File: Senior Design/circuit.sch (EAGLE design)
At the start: 24 parts, among them IC1 74HC164N, IC2 ATMEGA328P, IC3 ATTINY24A, Q1 16 MHz

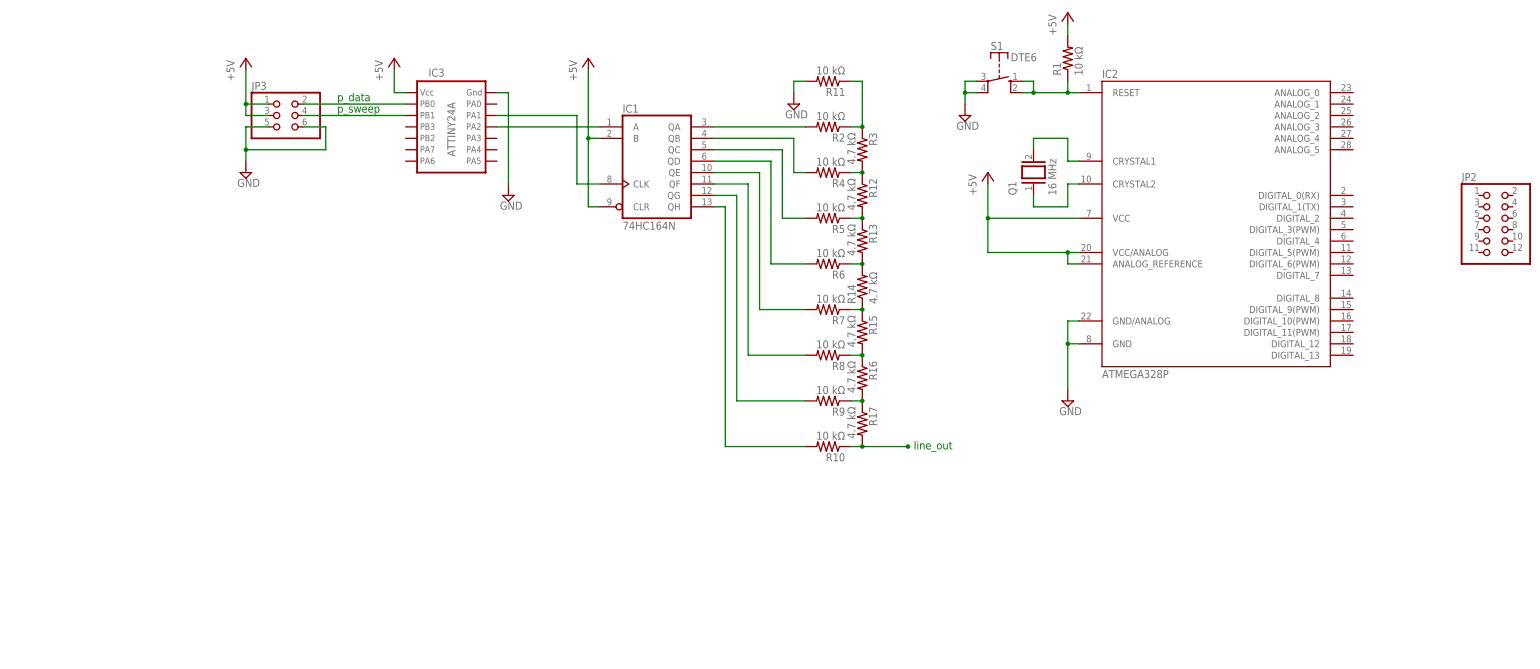
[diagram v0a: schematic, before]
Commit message: working on senior design PCB
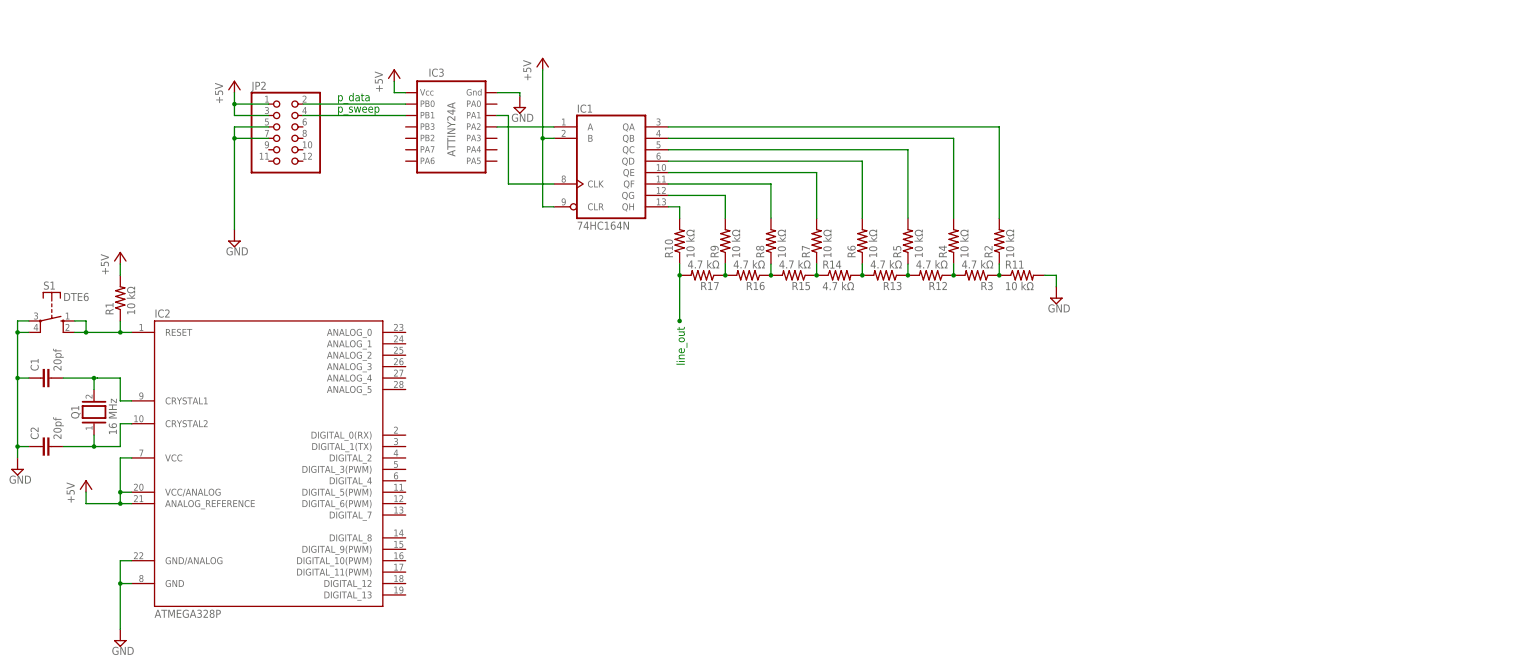
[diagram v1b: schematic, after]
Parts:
- removed JP3: (no value), pinhead:PINHD-2X3
- added C1, C2: 20pf, rcl:C-EU025-024X044
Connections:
- net +5V: now also JP2.1, JP2.3; no longer JP3.1, JP3.3
- net GND: now also C1.1, C2.1, JP2.5, JP2.7; no longer JP3.5, JP3.6
- net N$1: now also JP2.4; no longer JP3.4
- net N$2: now also JP2.2; no longer JP3.2
- net N$5: now also C1.2
- net N$6: now also C2.2
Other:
- moved on the sheet: IC1, IC2, JP2, Q1, R1, R10, R11, R12, R13, R14, R15, R16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
